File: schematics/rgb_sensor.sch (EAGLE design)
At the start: 7 parts, among them IC2 MEGA8-P

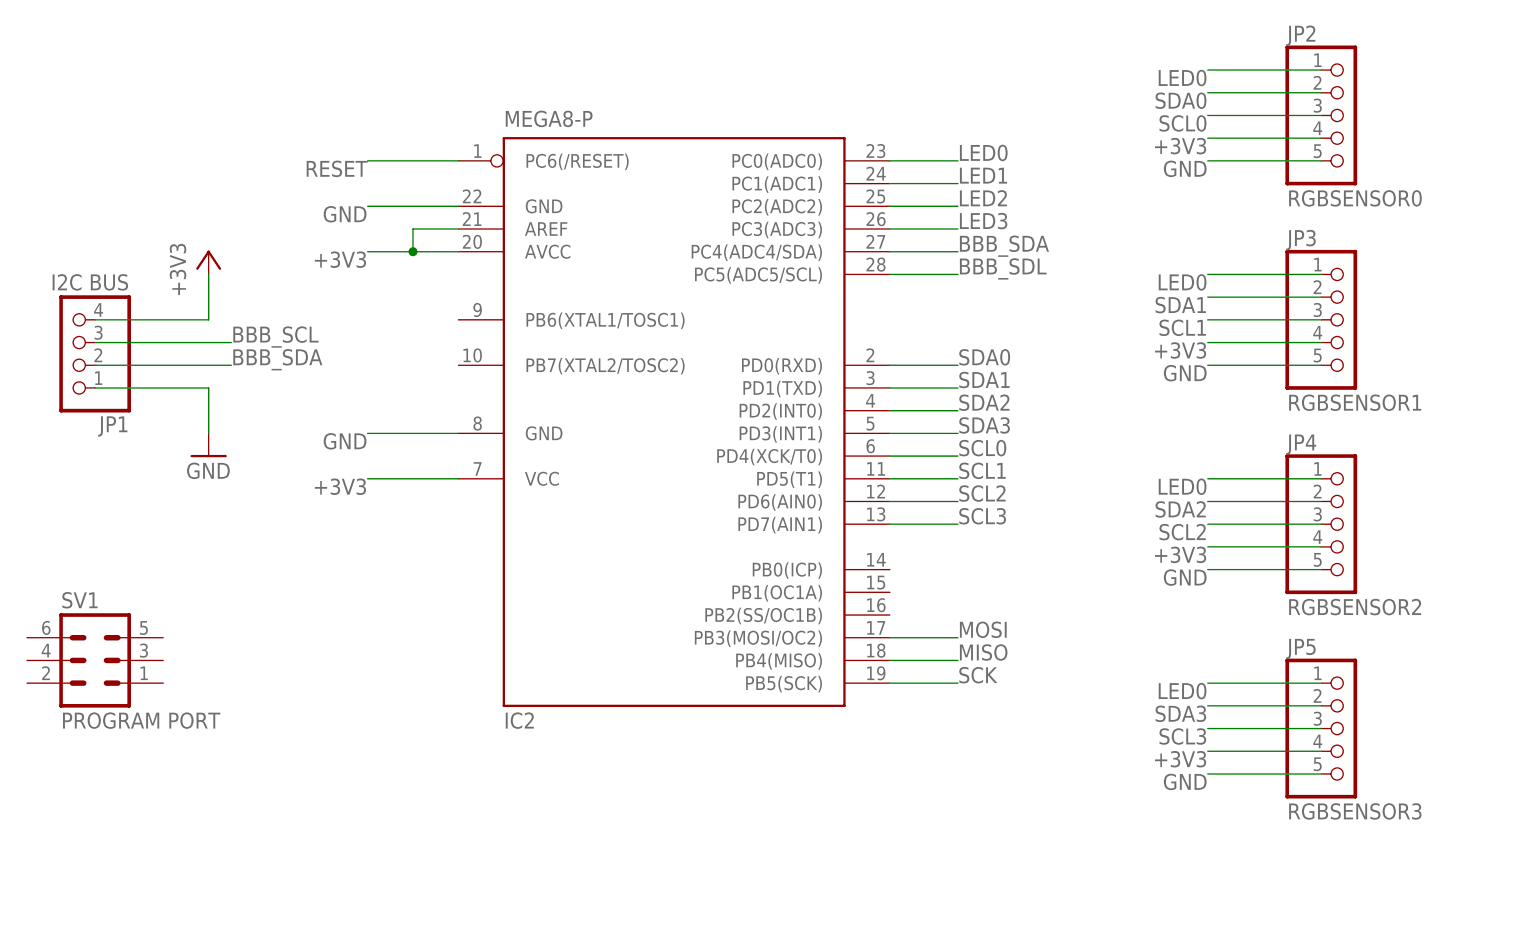
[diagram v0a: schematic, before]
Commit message: RGB Color Sensor Array Board Finalized to be Printed
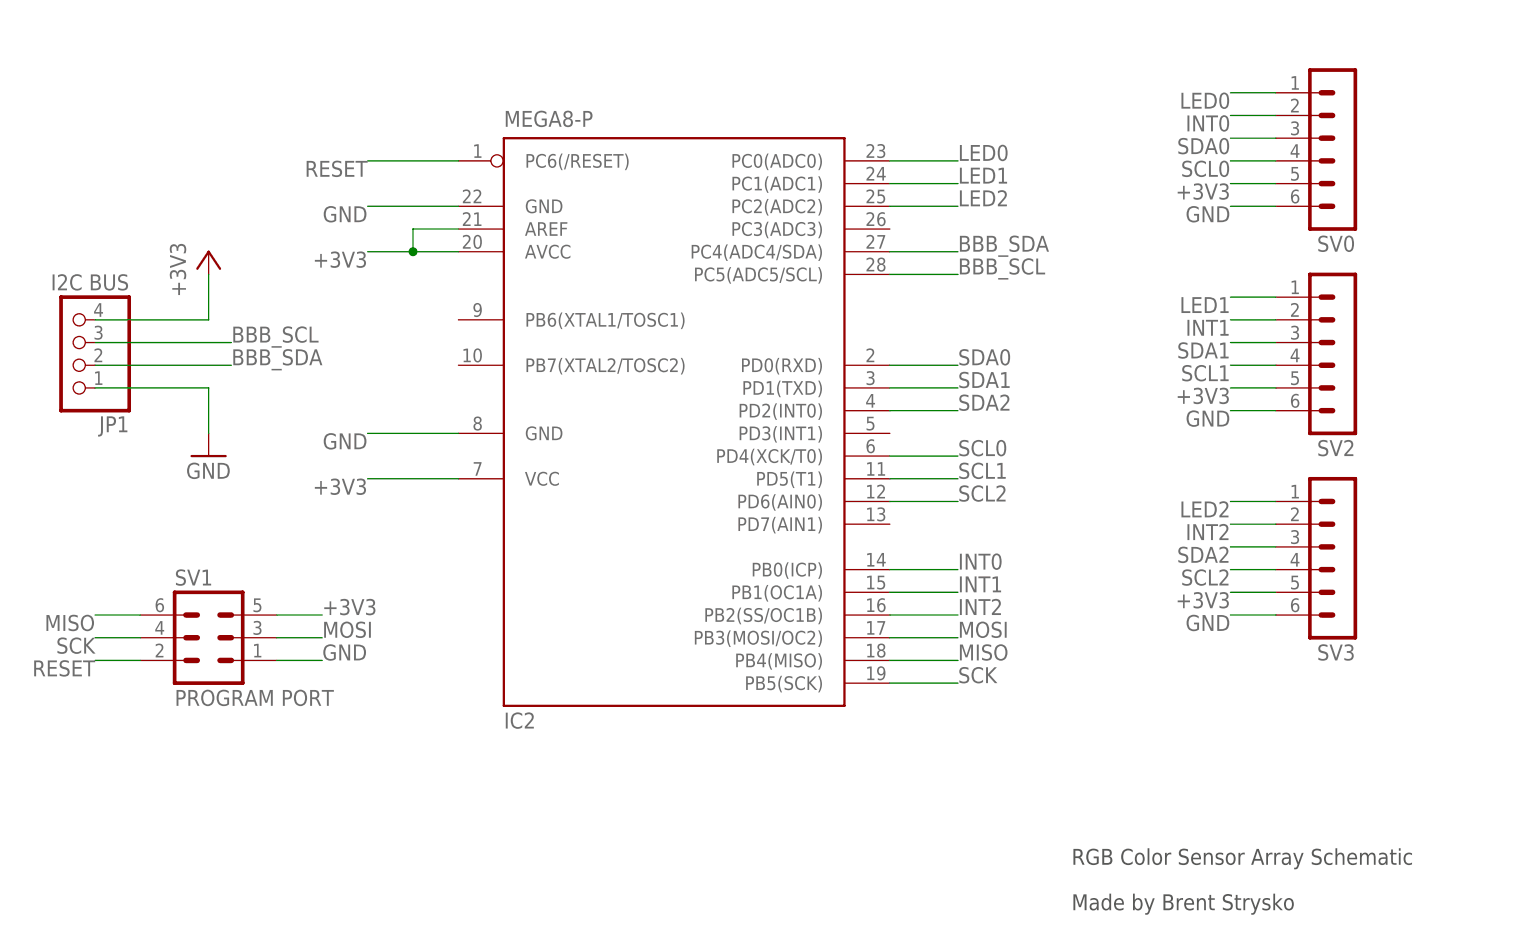
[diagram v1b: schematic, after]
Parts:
- removed JP2: RGBSENSOR0, pinhead:PINHD-1X5
- removed JP3: RGBSENSOR1, pinhead:PINHD-1X5
- removed JP4: RGBSENSOR2, pinhead:PINHD-1X5
- removed JP5: RGBSENSOR3, pinhead:PINHD-1X5
- added SV0, SV2, SV3: (no value), con-lstb:MA06-1
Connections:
- removed net BBB_SDL: IC2.PC5(ADC5/SCL)
- removed net LED3: IC2.PC3(ADC3)
- removed net SCL3: IC2.PD7(AIN1), JP5.3
- removed net SDA3: IC2.PD3(INT1), JP5.2
- new net INT0: IC2.PB0(ICP), SV0.2
- new net INT1: IC2.PB1(OC1A), SV2.2
- new net INT2: IC2.PB2(SS/OC1B), SV3.2
- net +3V3: now also SV0.5, SV1.5, SV2.5, SV3.5; no longer JP2.4, JP3.4, JP4.4, JP5.4
- net BBB_SCL: now also IC2.PC5(ADC5/SCL)
- net GND: now also SV0.6, SV1.1, SV2.6, SV3.6; no longer JP2.5, JP3.5, JP4.5, JP5.5
- net LED0: now also SV0.1; no longer JP2.1, JP3.1, JP4.1, JP5.1
- net LED1: now also SV2.1
- net LED2: now also SV3.1
- net MISO: now also SV1.6
- net MOSI: now also SV1.3
- net RESET: now also SV1.2
- net SCK: now also SV1.4
- net SCL0: now also SV0.4; no longer JP2.3
- net SCL1: now also SV2.4; no longer JP3.3
- net SCL2: now also SV3.4; no longer JP4.3
- net SDA0: now also SV0.3; no longer JP2.2
- net SDA1: now also SV2.3; no longer JP3.2
- net SDA2: now also SV3.3; no longer JP4.2
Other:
- note added: "Made by Brent Strysko"
- note added: "RGB Color Sensor Array Schematic"
- moved on the sheet: SV1
